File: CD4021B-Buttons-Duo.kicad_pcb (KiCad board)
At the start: 2 copper layers, 100 x 50 mm, 50 parts, among them J1 2.54, J10 JST XH, J11 JST XH, J12 JST XH, J13 JST XH, J14 JST XH, J15 JST XH, J16 JST XH, J17 JST XH, J18 3.5, J2 JST XH, J3 JST XH, J4 JST XH, J5 JST XH, J6 JST XH, J7 JST XH, J8 JST XH, J9 JST XH, Q1 IRF5806, Q2 IRF5806, Q3 IRF5806, Q4 IRF5806, Q5 IRF5806, Q6 IRF5806, Q7 IRF5806, Q8 IRF5806, U1 CD4021BM, U2 CD4021BM, U3 TPIC6C595D

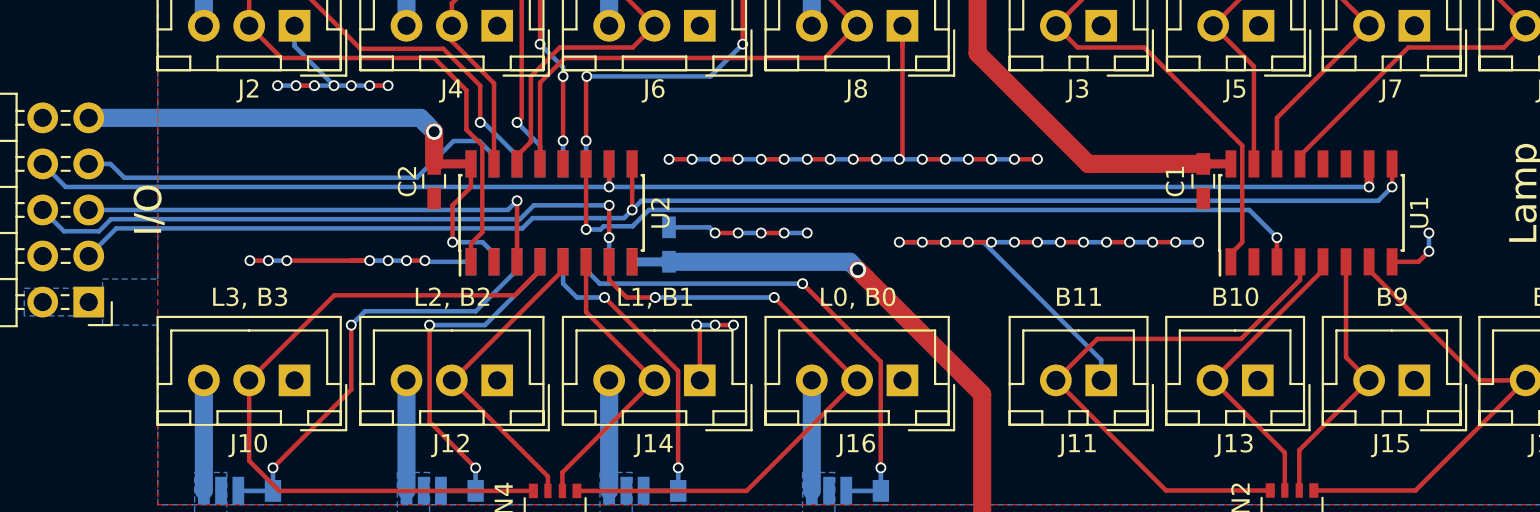
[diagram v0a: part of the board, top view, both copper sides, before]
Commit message: Cosmetic
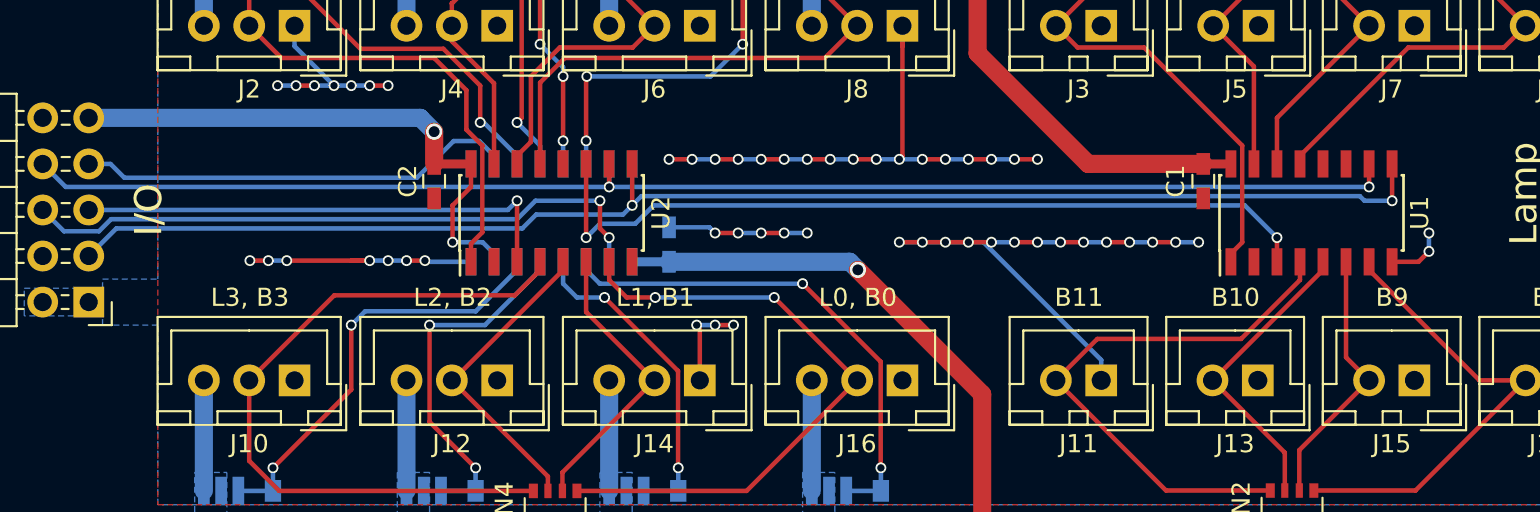
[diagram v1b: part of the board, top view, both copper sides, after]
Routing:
- net /CHAIN: track 44.1 -> 45.0 mm
